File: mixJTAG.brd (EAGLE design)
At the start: 100 x 83.8 mm, 88 parts, among them J1 PLUG-A, J10 CON_HEADER_1X08-PTH, J11 CON_HEADER_2X02-PTH, J12 CON_HEADER_1X08-PTH, J13 CON_HEADER_1X08-PTH, J2 CON_HEADER_1X03-PTH, J3 CON_HEADER_2X08, J4 CON_HEADER_2X10-PTH, J5 CON_HEADER_1X08-PTH, J6 CON_HEADER_1X08-PTH, J7 CON_HEADER_1X08-PTH, J8 CON_HEADER_1X08-PTH, J9 CON_HEADER_1X08-PTH, U1 SRV05-4, U10 74244DW, U11 74244DW, U12 74244DW, U13 74244DW, U2 93LC56B, U3 FT2232HLLQFP, U4 TC2117-800MA, U5 XC2C32A-6VQ44C, U6 SRV05-4, U7 SRV05-4, U8 SRV05-4, U9 SRV05-4, X1 12MHz

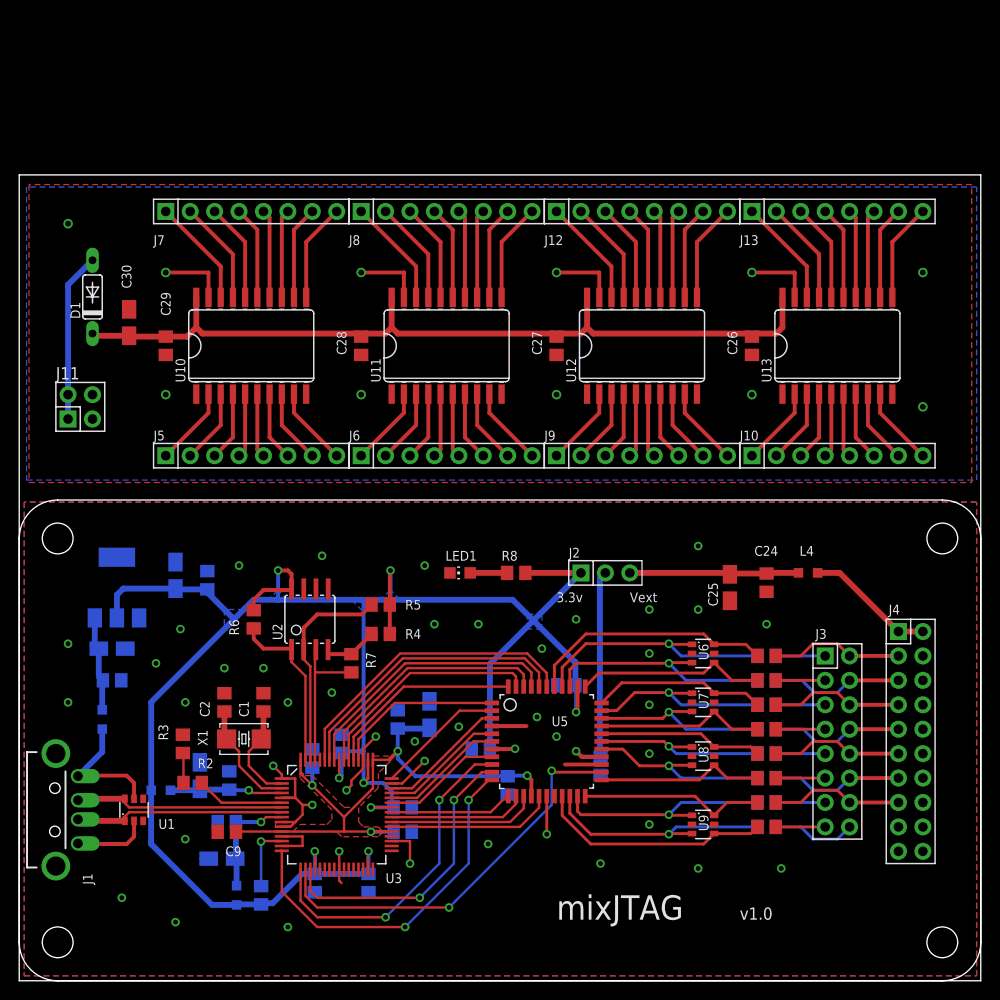
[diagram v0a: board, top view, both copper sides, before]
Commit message: more output
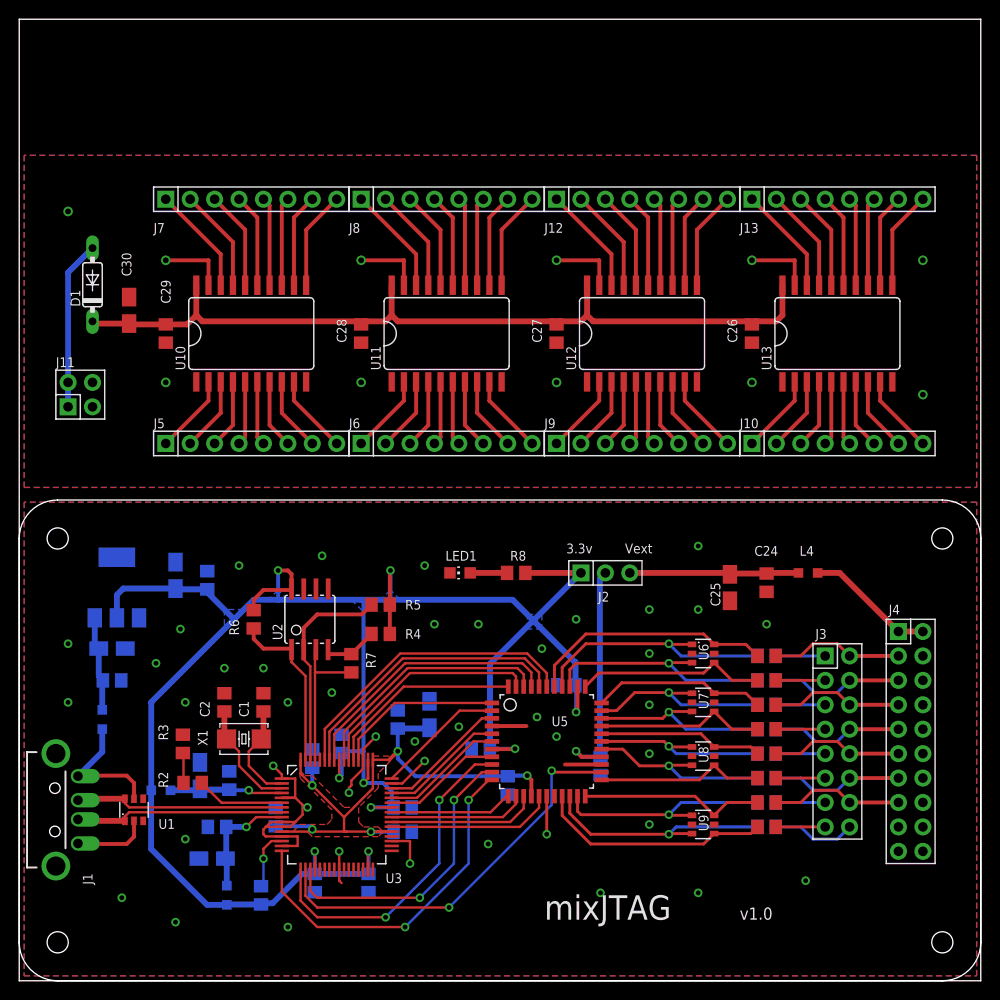
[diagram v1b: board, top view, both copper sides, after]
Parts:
- moved C9 5.30 mm to (26.7, 17.0), flipped to the bottom, turned to 90 degrees
- moved J10 1.27 mm to (85.1, 55.9)
- moved J11 1.27 mm to (6.35, 61.0)
- moved J5 1.27 mm to (24.1, 55.9)
- moved J6 1.27 mm to (44.5, 55.9)
- moved J9 1.27 mm to (64.8, 55.9)
- moved C26 1.27 mm to (76.2, 67.3)
- moved C27 1.27 mm to (55.9, 67.3)
- moved C28 1.27 mm to (35.6, 67.3)
- moved C29 1.27 mm to (15.2, 67.3)
- moved C30 1.27 mm to (11.4, 69.7)
- moved D1 1.27 mm to (7.62, 72.4)
- moved J12 1.27 mm to (64.8, 81.3)
- moved J13 1.27 mm to (85.1, 81.3)
- moved J7 1.27 mm to (24.1, 81.3)
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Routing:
- net GND: track 59.3 -> 63.2 mm
- net VPLL: track 11.7 -> 12.4 mm
- net +1V8: track 65.2 -> 64.6 mm, vias 4 -> 5
- net !RESET: track 6.85 -> 6.22 mm
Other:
- board size 100 x 83.8 mm -> 100 x 100 mm
- board text added: "VTref nTRST TDI TMS TCK RTCK TDO nSRST DBGRQ DBGACK"
- board text added: "Vsup GND GND GND GND GND GND GND GND GND"
